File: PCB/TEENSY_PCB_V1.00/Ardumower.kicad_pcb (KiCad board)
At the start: 2 copper layers, 169.8 x 97 mm, 50 parts, among them J1 ODO_Left, J10 Sonar_R, J11 Cutter, J12 Sonar_L, J13 P_Right, J14 Buzzer, J15 Button, J16 Power_Board, J19 P_Left, J2 I2C2_0, J25 5V IN, J29 3.3V IN, J3 I2C0_0, J30 I2C1_0, J31 Ser3, J4 I2C1_1, J5 Bumper, J6 ODO_Right, J7 Motor_Right1, J8 Motor_Left1, J9 Rain, U1 DOIT-ESP32-DEVKIT-V1, U2 GY-521, U3 Teensy4.1

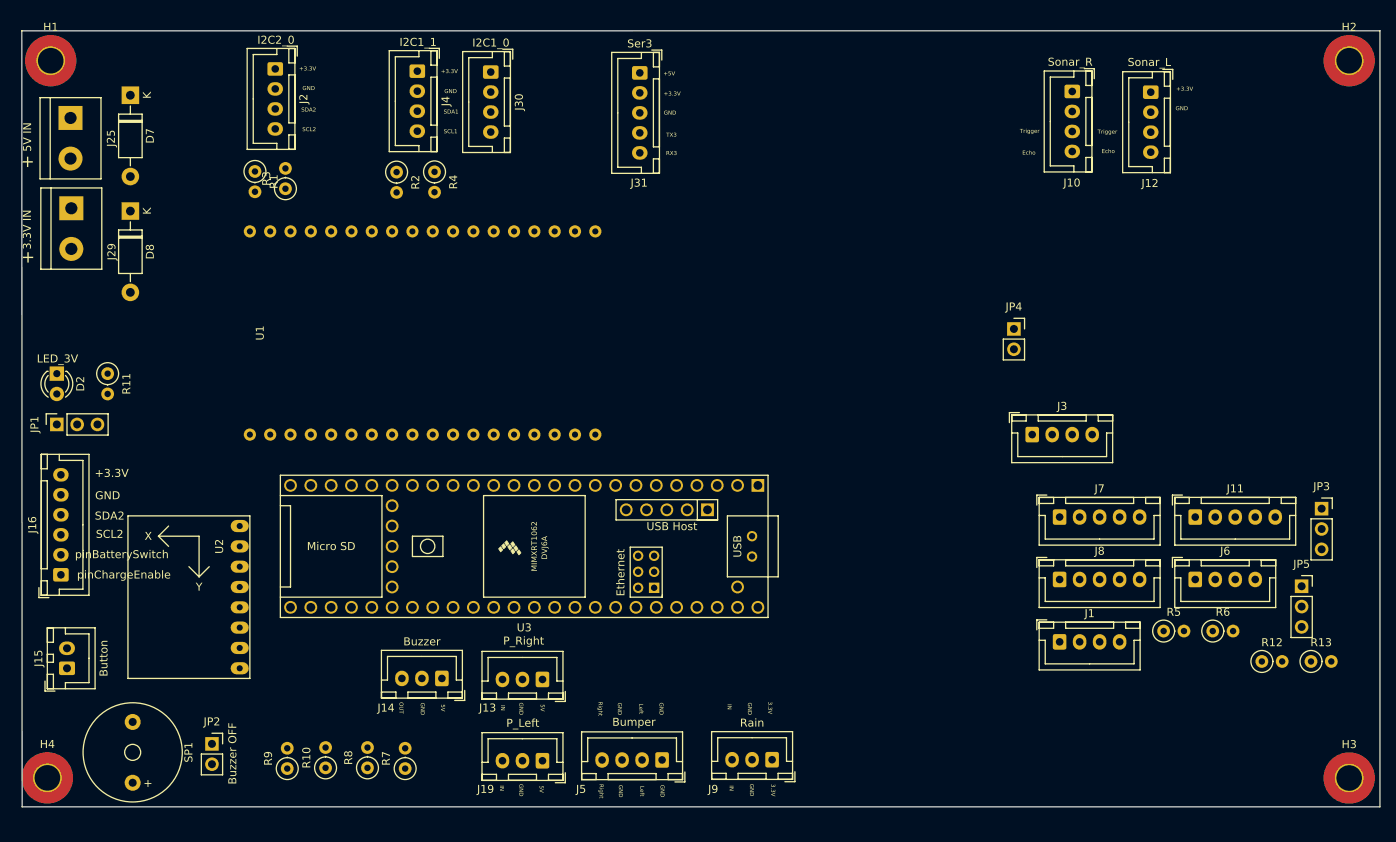
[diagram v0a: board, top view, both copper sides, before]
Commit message: test
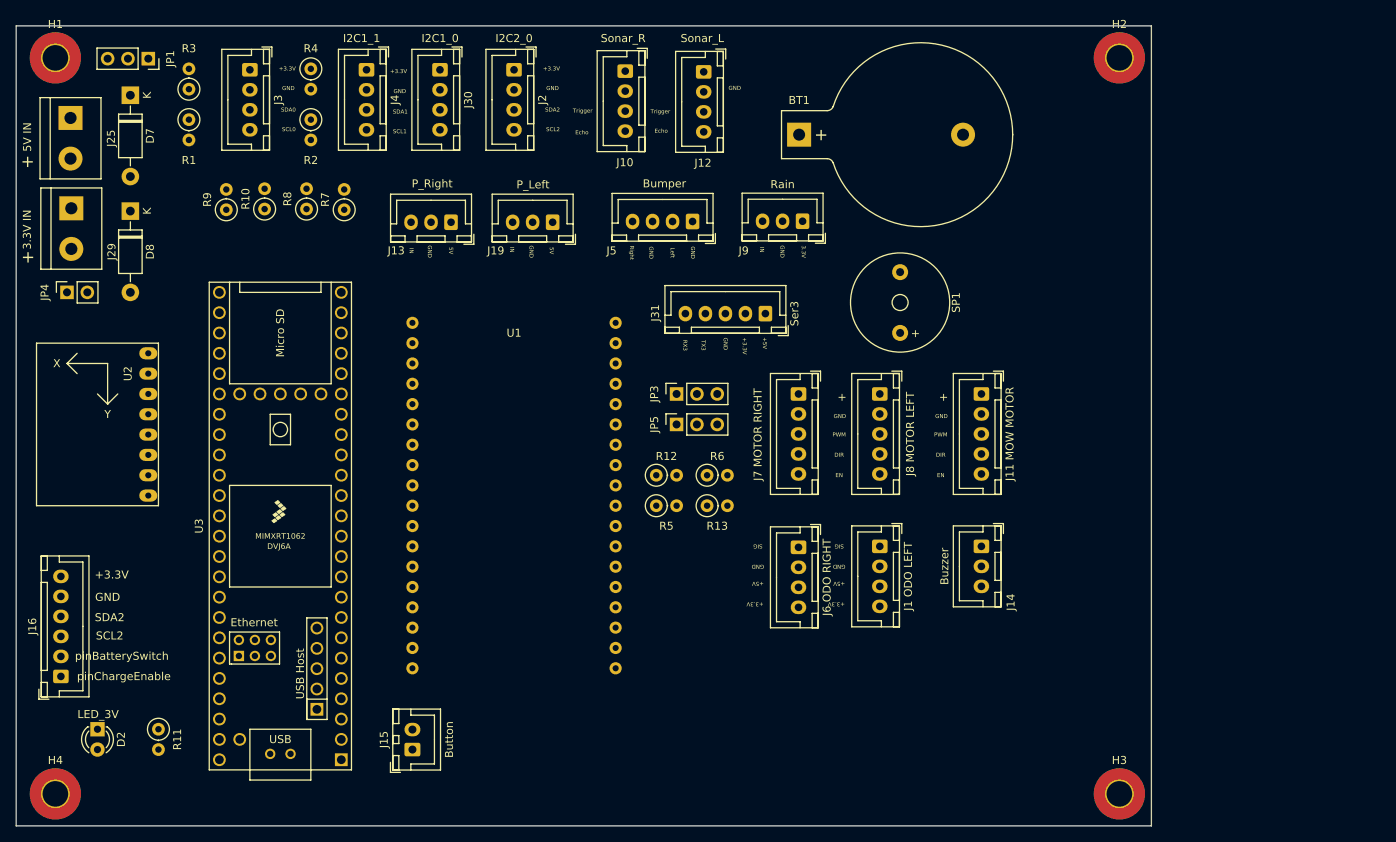
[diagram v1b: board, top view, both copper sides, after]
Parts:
- removed JP2: Buzzer OFF, Connector_PinSocket_2.54mm:PinSocket_1x02_P2.54mm_Vertical
- added BT1: Battery_Cell, Battery:BatteryHolder_Keystone_103_1x20mm, F.Cu at (136.0, 47.6)
- J1 ODO LEFT: renamed from J1
- J11 MOW MOTOR: renamed from J11
- J6 ODO RIGHT: renamed from J6
- J7 MOTOR RIGHT: renamed from J7
- J8 MOTOR LEFT: renamed from J8
- moved JP4 118.5 mm to (44.5, 67.3), turned to 90 degrees
- moved SP1 111.2 mm to (148.6, 68.6)
- moved J3 107.9 mm to (67.3, 39.5), turned to 270 degrees
- moved JP3 81.9 mm to (120.7, 80.0), turned to 90 degrees
- moved JP5 80.7 mm to (120.7, 83.8), turned to 90 degrees
- moved R12 79.2 mm to (118.1, 90.2)
- moved R13 78.0 mm to (124.5, 94.0)
- moved R10 70.3 mm to (69.2, 56.9)
- moved R7 70.3 mm to (79.1, 57.0)
- moved R8 70.3 mm to (74.4, 56.9)
- moved R9 70.3 mm to (64.4, 57.0)
- moved J14 69.4 mm to (158.8, 99.1), turned to 270 degrees
- moved J5 67.4 mm to (122.6, 58.5)
- moved J9 67.4 mm to (136.4, 58.4)
- moved J19 67.3 mm to (105.2, 58.5)
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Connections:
- J10 pad 3: (no net) -> pinSonarRightTrigger
- J10 pad 4: (no net) -> pinSonarRightEcho
- J12 pad 3: (no net) -> pinSonarLeftTrigger
- J12 pad 4: (no net) -> pinSonarLeftEcho
- SP1 pad 2: Net-(JP2-Pad2) -> pinBuzzer
- U3 pad 18: (no net) -> pinSonarLeftEcho
- U3 pad 19: (no net) -> pinSonarRightEcho
- U3 pad 20: (no net) -> pinSonarLeftTrigger
- U3 pad 21: (no net) -> pinSonarRightTrigger
- U3 pad 50: (no net) -> Net-(BT1-Pad1)
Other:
- board size 169.8 x 97 mm -> 141.9 x 100 mm
- board text added: "DIR"
- board text added: "EN"
- board text added: "PWM"
- board text added: "SCL0"
- board text added: "SDA0"
- board text added: "SIG"
- board text removed: "OUT"
